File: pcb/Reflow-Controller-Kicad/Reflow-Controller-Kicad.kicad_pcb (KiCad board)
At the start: 2 copper layers, 58.4 x 67.3 mm, 88 parts, among them J1 , J10 , J2 USB_C_Receptacle_USB2.0, J3 , J4 , J5 , J6 , J7 , J8 , J9 Servo, Q1 IRLML2502, Q2 IRLML2502, Q3 IRLML2502, Q4 IRLML2502, Q5 IRLML2502, SW1 SW_Push_SPDT, SW2 RST, SW3 BOOT, U1 ESP32-S2-WROVER, U2 MAX6675, U3 MAX6675, U4 MIC5219-3.3YM5

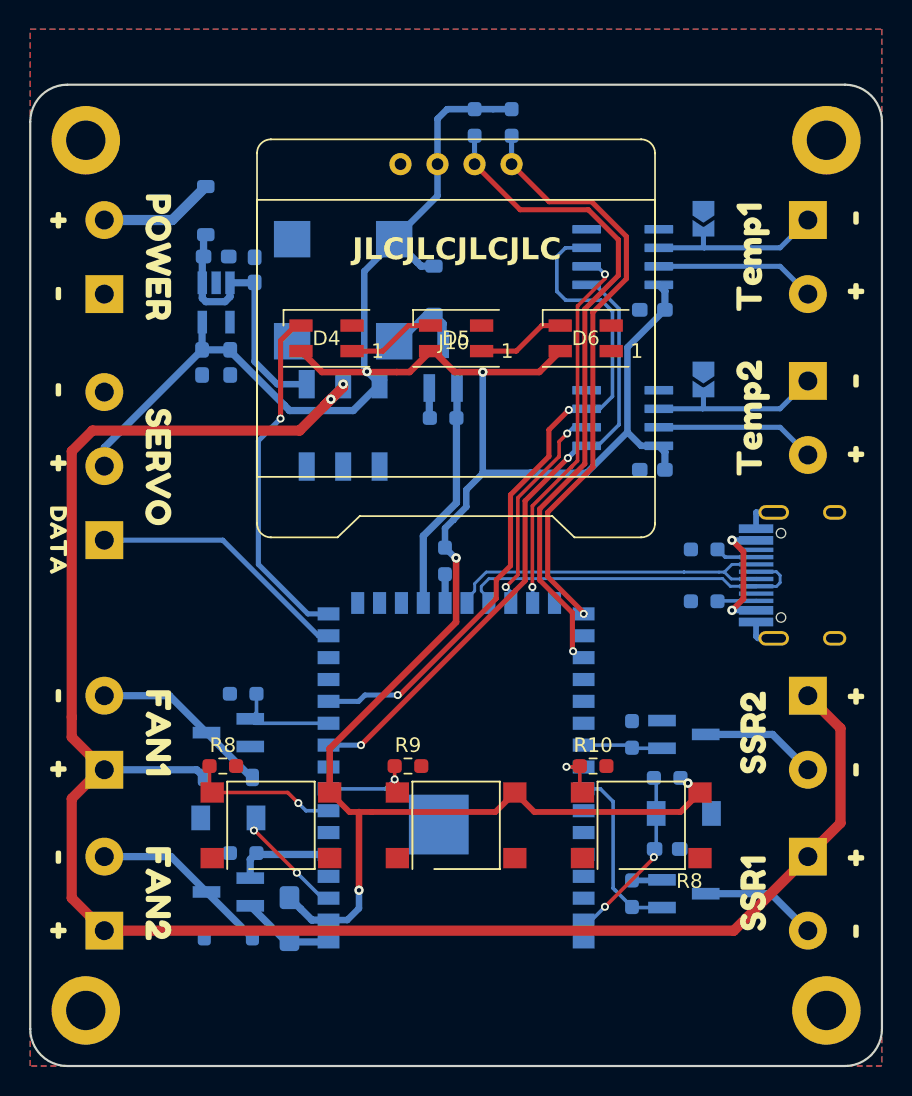
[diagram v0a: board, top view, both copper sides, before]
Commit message: Update
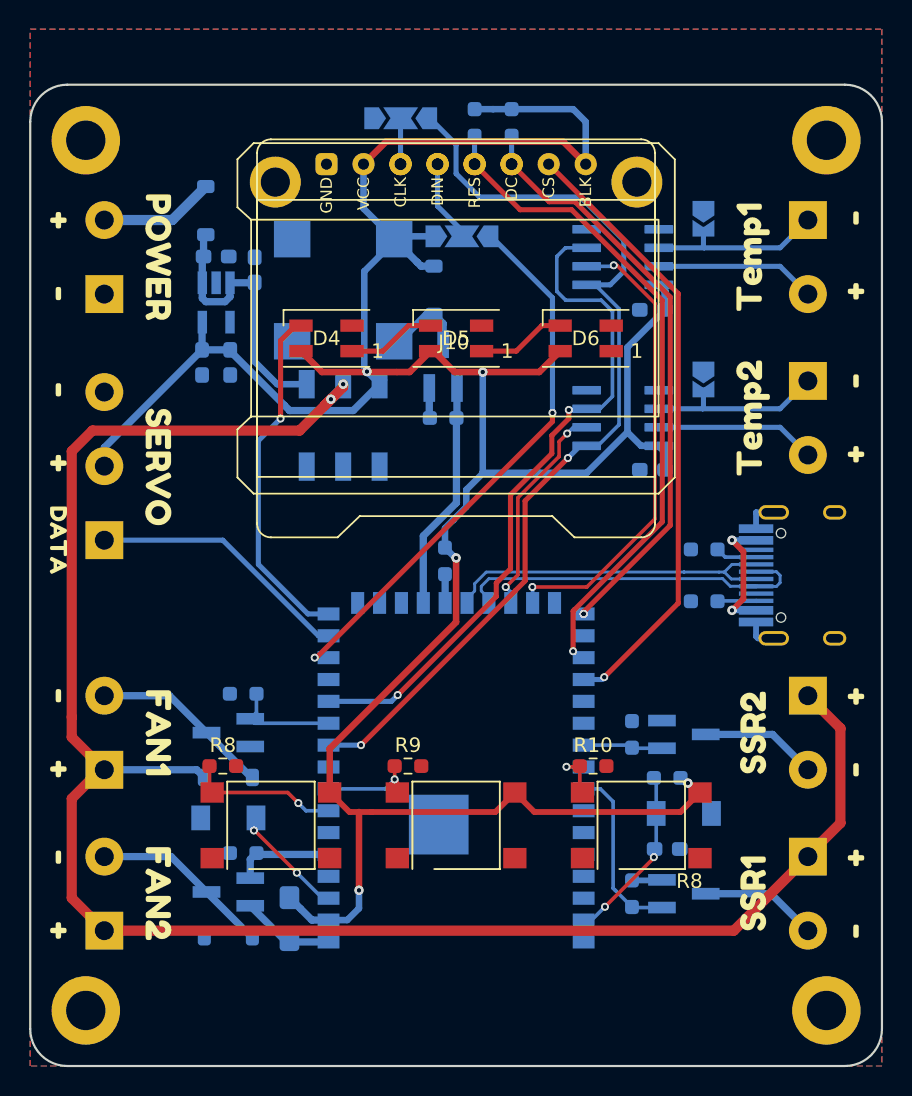
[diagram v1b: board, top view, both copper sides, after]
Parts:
- added J11: Conn_01x08, footprint:0.96_TFT_Display_ST77335S, F.Cu at (101.6, 66.8)
- added JP3: , Jumper:SolderJumper-3_P2.0mm_Open_TrianglePad1.0x1.5mm, B.Cu at (102.0, 61.2)
- added JP4: , Jumper:SolderJumper-3_P2.0mm_Open_TrianglePad1.0x1.5mm, B.Cu at (97.8, 53.1)
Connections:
- J10 pad 1: GND -> Net-(J10-Pin_1)
- J10 pad 2: +3.3V -> Net-(J10-Pin_2)
- U1 pad 30: unconnected-(U1-IO36-Pad30) -> CS_DISPLAY
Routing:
- net CS_DISPLAY: track 0.00 -> 42.5 mm, vias 0 -> 1
- net MOSI: track 0.00 -> 38.4 mm, vias 0 -> 2
- net CLK: track 43.1 -> 66.1 mm
- net +3.3V: track 182.0 -> 203.3 mm
- net CS_MAX1: track 26.2 -> 32.0 mm
- net Net-(J10-Pin_2): track 0.00 -> 5.64 mm
- net Net-(J10-Pin_1): track 0.00 -> 3.15 mm
- net SDA: track 41.0 -> 40.8 mm, vias 1 -> 2
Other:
- board text removed: "JLCJLCJLCJLC"
